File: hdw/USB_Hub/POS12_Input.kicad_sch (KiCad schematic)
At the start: 21 parts

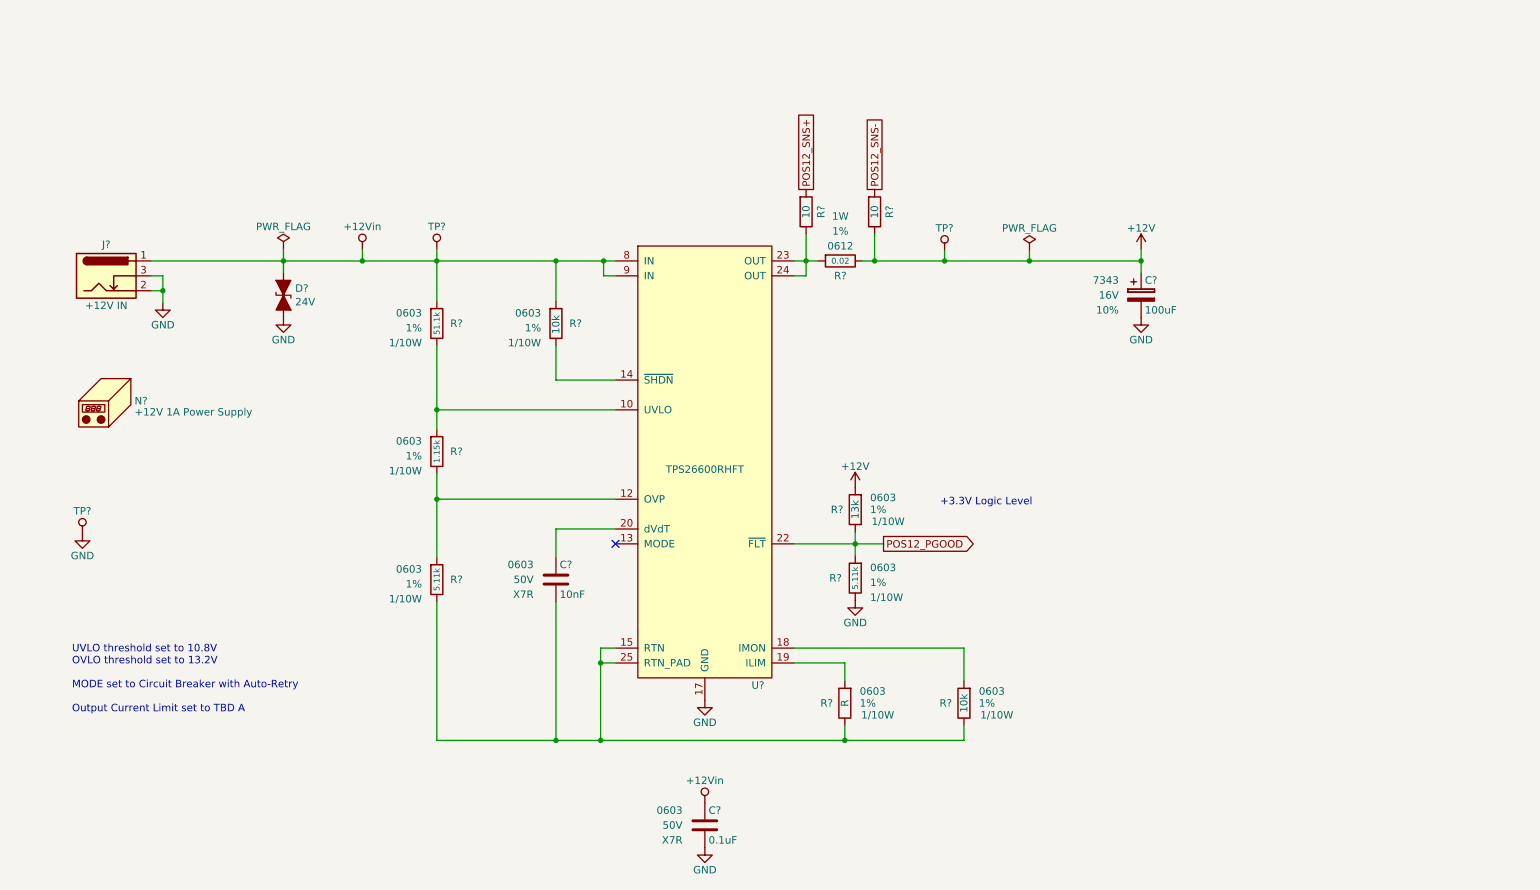
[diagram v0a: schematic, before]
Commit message: schematic progress
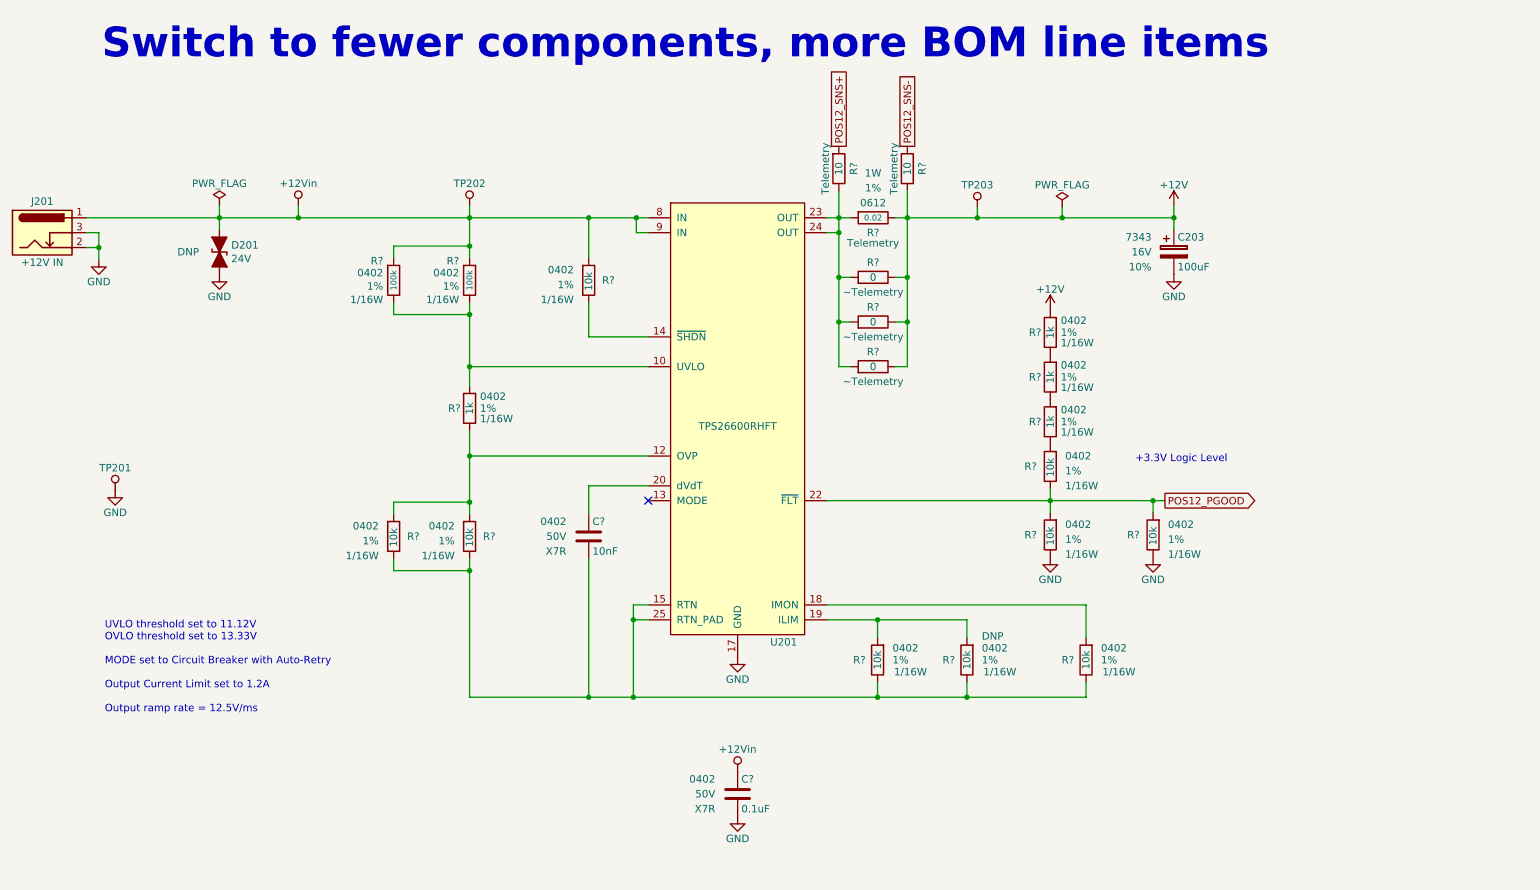
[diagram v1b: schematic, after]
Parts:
- removed C?: 0.1uF, Capacitors_SMD:C_0603, symbol Custom_Library:C_Custom
- removed C?: 100uF, Capacitors_Tantalum_SMD:CP_Tantalum_Case-X_EIA-7343-43_Reflow, symbol Custom_Library:CP_Tant_Custom
- removed C?: 10nF, Capacitors_SMD:C_0603, symbol Custom_Library:C_Custom
- removed D?: 24V, Diodes_SMD:D_SMA, symbol Device:D_TVS_ALT
- removed J?: +12V IN, Connectors:BARREL_JACK, symbol Connector:Barrel_Jack_Switch
- removed N?: +12V 1A Power Supply, symbol Mechanical:Housing
- removed R?: 1.15k, Resistors_SMD:R_0603, symbol Custom_Library:R_Custom
- removed R?: 51.1k, Resistors_SMD:R_0603, symbol Custom_Library:R_Custom
- removed R? (x2): 5.11k, Resistors_SMD:R_0603, symbol Custom_Library:R_Custom
- removed R? (x2): 10k, Resistors_SMD:R_0603, symbol Custom_Library:R_Custom
- removed R?: 0.02, Resistors_SMD:R_0612, symbol Custom_Library:R_Custom
- removed R? (x2): 10, Resistors_SMD:R_0603, symbol Custom_Library:R_Custom
- removed R?: 13k, Resistors_SMD:R_0603, symbol Custom_Library:R_Custom
- removed R?: R, Resistors_SMD:R_0603, symbol Custom_Library:R_Custom
- removed TP? (x2): TP_Pad, Custom Footprints Library:Test_Point, symbol Custom_Library:TP_Pad
- removed TP?: TP, Pin_Headers:Pin_Header_Angled_1x01_Pitch2.54mm, symbol Custom_Library:TP
- removed U?: TPS26600RHFT, Housings_DFN_QFN:QFN-24-1EP_4x5mm_Pitch0.5mm, symbol Custom_Library:TPS26600RHFT
- added C203: 100uF, Capacitors_Tantalum_SMD:CP_Tantalum_Case-X_EIA-7343-43_Reflow, symbol Custom_Library:CP_Tant_Custom
- added C?: 0.1uF, Capacitors_SMD:C_0402, symbol Custom_Library:C_Custom
- added C?: 10nF, Capacitors_SMD:C_0402, symbol Custom_Library:C_Custom
- added D201: 24V, Diodes_SMD:D_SMA, symbol Device:D_TVS_ALT
- added J201: +12V IN, Connectors:BARREL_JACK, symbol Connector:Barrel_Jack_Switch
- added R? (x2): 100k, Resistors_SMD:R_0402, symbol Custom_Library:R_Custom
- added R? (x9): 10k, Resistors_SMD:R_0402, symbol Custom_Library:R_Custom
- added R? (x3): 0, Resistors_SMD:R_0402, symbol Custom_Library:R_Custom
- added R? (x2): 10, Resistors_SMD:R_0402, symbol Custom_Library:R_Custom
- added R? (x4): 1k, Resistors_SMD:R_0402, symbol Custom_Library:R_Custom
- added R?: 0.02, Resistors_SMD:R_0612, symbol Custom_Library:R_Custom
- added TP201: TP, Pin_Headers:Pin_Header_Angled_1x01_Pitch2.54mm, symbol Custom_Library:TP
- added TP202, TP203: TP, Custom Footprints Library:Test_Point, symbol Custom_Library:TP_Pad
- added U201: TPS26600RHFT, Housings_DFN_QFN:QFN-24-1EP_4x5mm_Pitch0.5mm, symbol Custom_Library:TPS26600RHFT
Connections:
- net +12V: now also C203.1, R?.1, R?.2, R?.2, R?.2, R?.2, R?.2, TP203.1 (TP)
- net +12Vin: now also C?.1, D201.1 (A1), J201.1, R?.1, R?.1, R?.1, TP202.1 (TP), U201.8 (IN), U201.9 (IN)
- net GND: now also C203.2, C?.2, D201.2 (A2), J201.2, J201.3, R?.2, R?.2, TP201.1 (TP), U201.17 (GND)
- net POS12_PGOOD: now also R?.1, R?.1, R?.2, U201.22 (~{FLT})
- net POS12_SNS+: now also R?.1
- net POS12_SNS-: now also R?.1
- new net: R?.1, R?.2, R?.2, U201.10 (UVLO)
- new net: R?.2, U201.14 (~{SHDN})
- new net: R?.1, R?.2 (x3)
- new net: R?.1, R?.1, R?.2, U201.12 (OVP)
- new net: C?.2, R?.2, R?.2, R?.2, R?.2, R?.2, U201.15 (RTN), U201.25 (RTN_PAD)
- new net: R?.1, R?.1, R?.1, R?.1, R?.2, U201.23 (OUT), U201.24 (OUT)
- new net: R?.1, U201.18 (IMON)
- new net: R?.1, R?.1, U201.19 (ILIM)
- new net: C?.1, U201.20 (dVdT)
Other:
- note added: "Switch to fewer components, more BOM line items"
- note added: "UVLO threshold set to 11.12V OVLO threshold set to 13.33V MODE set to Circuit Breaker with Auto-Retry Output Current Limit set to 1.2A Output ramp rate = 12.5V/ms"
- note removed: "UVLO threshold set to 10.8V OVLO threshold set to 13.2V MODE set to Circuit Breaker with Auto-Retry Output Current Limit set to TBD A"
